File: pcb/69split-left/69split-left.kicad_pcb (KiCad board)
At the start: 2 copper layers, 157.5 x 108.9 mm, 94 parts, among them J1 USB_C_Receptacle_USB2.0_16P, J2 Conn_02x03_Odd_Even, J3 USB_C_Receptacle_USB2.0_16P, J4 Conn_01x09_Socket, SW1 SW_Push, SW10 SW_Push, SW11 SW_Push, SW12 SW_Push, SW13 SW_Push, SW14 SW_Push, SW15 SW_Push, SW16 SW_Push, SW17 SW_Push, SW18 SW_Push, SW19 SW_Push, SW2 SW_Push, SW20 SW_Push, SW21 SW_Push, SW22 SW_Push, SW23 SW_Push, SW24 SW_Push, SW25 SW_Push, SW26 SW_Push, SW27 SW_Push, SW28 SW_Push, SW29 SW_Push, SW3 SW_Push, SW30 SW_Push, SW31 SW_Push, SW4 SW_Push, SW5 SW_Push, SW6 SW_Push, SW7 SW_Push, SW8 SW_Push, SW9 SW_Push, U1 ATmega32U4-AU, U2 TLV76133DCY, Y1 Crystal

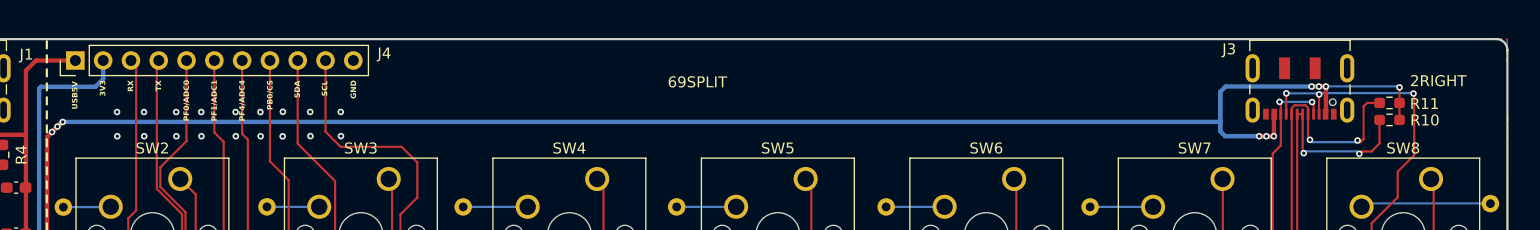
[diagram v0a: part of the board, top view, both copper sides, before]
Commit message: Finished design and layout?
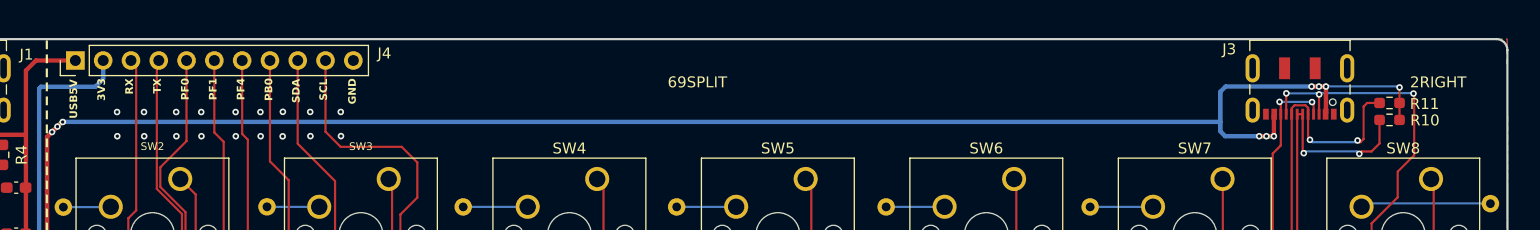
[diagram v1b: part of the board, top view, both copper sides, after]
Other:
- board text added: "PB0"
- board text added: "PF0"
- board text added: "PF1"
- board text added: "PF4"
- board text removed: "PB0/CS"
- board text removed: "PF0/ADC0"
- board text removed: "PF1/ADC1"
- board text removed: "PF4/ADC4"
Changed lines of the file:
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@@
 		(allow_soldermask_bridges_in_footprints no)
 		(tenting front back)
+		(grid_origin 59.6 143.14)
 		(pcbplotparams
 			(layerselection 0x00000000_00000000_55555555_5755f5ff)
@@
 		(tags "Cherry MX keyswitch 1.00u PCB")
 		(property "Reference" "SW2"
-			(at -2.54 -2.794 0)
+			(at -2.54 -2.974 0)
 			(layer "F.SilkS")
 			(effects
 				(font
-					(size 1 1)
-					(thickness 0.15)
+					(size 0.7 0.7)
+					(thickness 0.12)
 				)
 			)
@@
 		(tags "Cherry MX keyswitch 1.00u PCB")
 		(property "Reference" "SW3"
-			(at -2.54 -2.794 0)
+			(at -2.54 -2.974 0)
 			(layer "F.SilkS")
 			(effects
 				(font
-					(size 1 1)
-					(thickness 0.15)
+					(size 0.7 0.7)
+					(thickness 0.12)
 				)
 			)
@@
 		(layer "Edge.Cuts")
 	)
-	(gr_text "PB0/CS"
-		(at 99.5775 37.97 90)
+	(gr_text "PB0"
+		(at 99.5775 37.79 90)
 		(layer "F.SilkS" knockout)
 		(effects
 			(font
-				(size 0.5 0.5)
-				(thickness 0.1)
+				(size 0.7 0.7)
+				(thickness 0.12)
 				(bold yes)
 			)
@@
 	)
 	(gr_text "USB5V"
-		(at 81.745 38.08 90)
+		(at 81.745 37.9 90)
 		(layer "F.SilkS" knockout)
 		(effects
 			(font
-				(size 0.5 0.5)
-				(thickness 0.1)
+				(size 0.7 0.7)
+				(thickness 0.12)
 				(bold yes)
 			)
@@
 	)
 	(gr_text "GND"
-		(at 107.21 37.99 90)
+		(at 107.21 37.81 90)
 		(layer "F.SilkS" knockout)
 		(effects
 			(font
-				(size 0.5 0.5)
-				(thickness 0.1)
+				(size 0.7 0.7)
+				(thickness 0.12)
 				(bold yes)
 			)
@@
 		)
 	)
-	(gr_text "PF0/ADC0"
-		(at 91.935 37.97 90)
+	(gr_text "PF0"
+		(at 91.935 37.79 90)
 		(layer "F.SilkS" knockout)
 		(effects
 			(font
-				(size 0.5 0.5)
-				(thickness 0.1)
+				(size 0.7 0.7)
+				(thickness 0.12)
 				(bold yes)
 			)
@@
 		)
 	)
-	(gr_text "PF4/ADC4"
-		(at 97.03 37.97 90)
+	(gr_text "PF4"
+		(at 97.03 37.79 90)
 		(layer "F.SilkS" knockout)
 		(effects
 			(font
-				(size 0.5 0.5)
-				(thickness 0.1)
+				(size 0.7 0.7)
+				(thickness 0.12)
 				(bold yes)
 			)
@@
 	)
 	(gr_text "RX"
-		(at 86.84 38 90)
+		(at 86.84 37.82 90)
 		(layer "F.SilkS" knockout)
 		(effects
 			(font
-				(size 0.5 0.5)
-				(thickness 0.1)
+				(size 0.7 0.7)
+				(thickness 0.12)
 				(bold yes)
 			)
@@
 		)
 	)
-	(gr_text "PF1/ADC1"
-		(at 94.4825 37.97 90)
+	(gr_text "PF1"
+		(at 94.4825 37.79 90)
 		(layer "F.SilkS" knockout)
 		(effects
 			(font
-				(size 0.5 0.5)
-				(thickness 0.1)
+				(size 0.7 0.7)
+				(thickness 0.12)
 				(bold yes)
 			)
@@
 	)
 	(gr_text "SDA"
-		(at 102.08 38.03 90)
+		(at 102.08 37.85 90)
 		(layer "F.SilkS" knockout)
 		(effects
 			(font
-				(size 0.5 0.5)
-				(thickness 0.1)
+				(size 0.7 0.7)
+				(thickness 0.12)
 				(bold yes)
 			)
@@
 	)
 	(gr_text "2RIGHT"
-		(at 206.04 38.07 0)
+		(at 206.04 38.18 0)
 		(layer "F.SilkS" knockout)
 		(effects
@@
 	)
 	(gr_text "3V3"
-		(at 84.29 37.98 90)
+		(at 84.29 37.8 90)
 		(layer "F.SilkS" knockout)
 		(effects
 			(font
-				(size 0.5 0.5)
-				(thickness 0.1)
+				(size 0.7 0.7)
+				(thickness 0.12)
 				(bold yes)
 			)
@@
 	)
 	(gr_text "TX"
-		(at 89.3875 38 90)
+		(at 89.3875 37.82 90)
 		(layer "F.SilkS" knockout)
 		(effects
 			(font
-				(size 0.5 0.5)
-				(thickness 0.1)
+				(size 0.7 0.7)
+				(thickness 0.12)
 				(bold yes)
 			)
@@
 	)
 	(gr_text "SCL"
-		(at 104.58 38.03 90)
+		(at 104.58 37.85 90)
 		(layer "F.SilkS" knockout)
 		(effects
 			(font
-				(size 0.5 0.5)
-				(thickness 0.1)
+				(size 0.7 0.7)
+				(thickness 0.12)
 				(bold yes)
 			)
